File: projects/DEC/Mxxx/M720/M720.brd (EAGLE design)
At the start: 125.7 x 62.2 mm, 38 parts, among them Q1 2N3009, Q2 2N3009, Q3 2N3009, Q4 2N3009, Q5 2N3009, Q6 2N3009

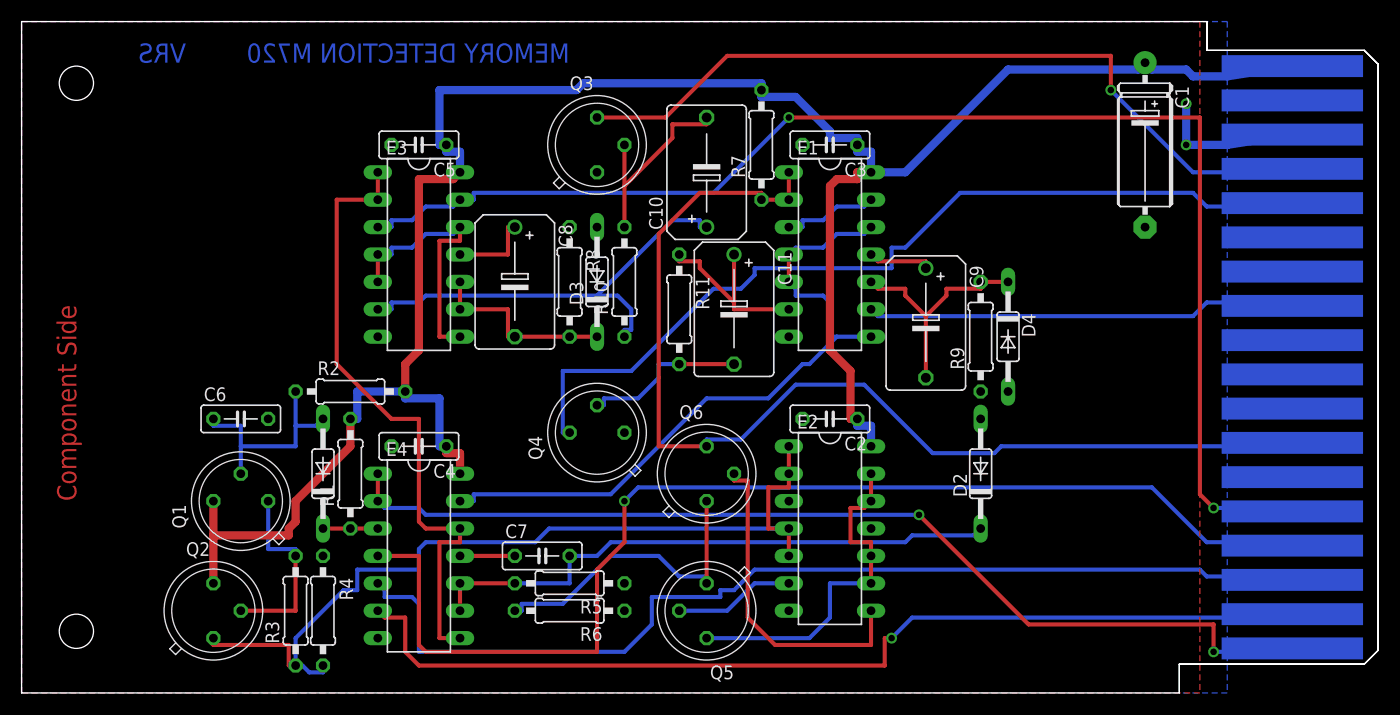
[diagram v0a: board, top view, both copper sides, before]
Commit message: Walk the project tree, making things pass current design rules.
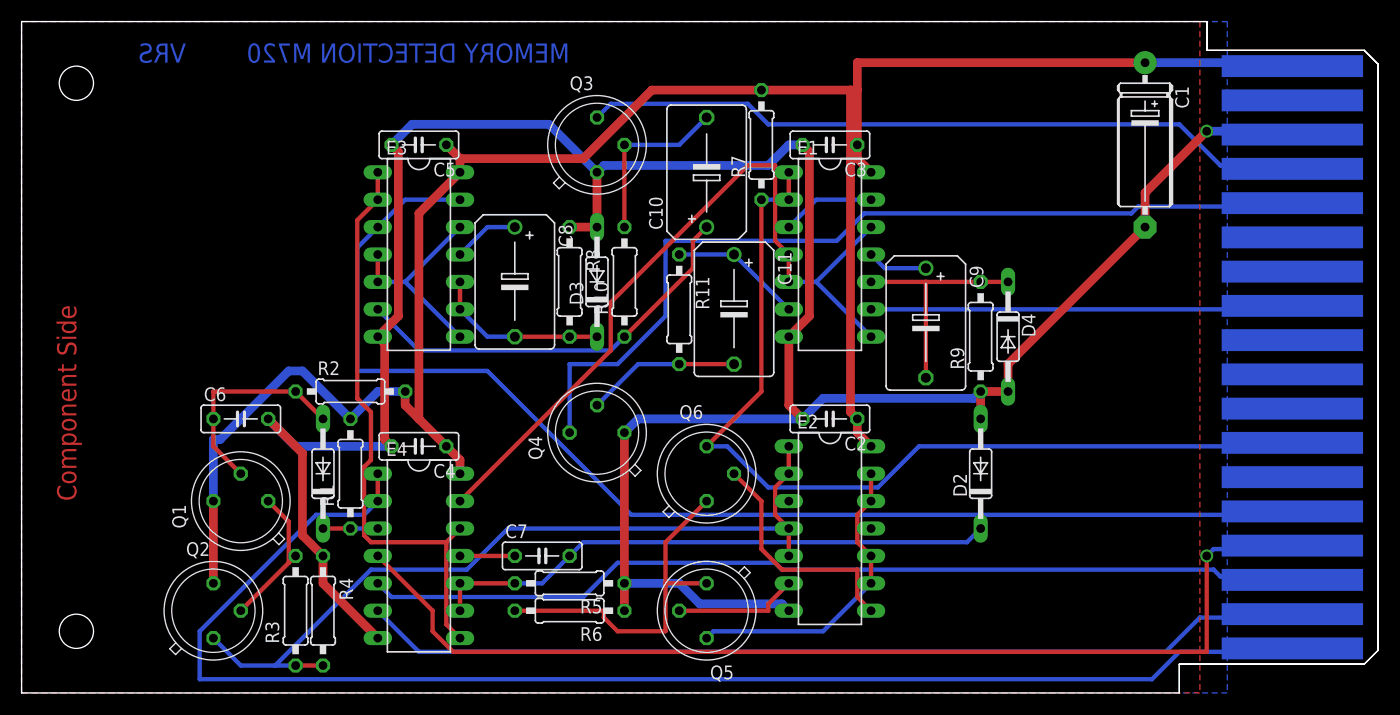
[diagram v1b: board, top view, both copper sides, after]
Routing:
- net GND: track 19.9 -> 255.2 mm, vias 2 -> 1
- net MEM_START: track 94.6 -> 131.0 mm, vias 2 -> 0
- net N$8: track 100.9 -> 87.6 mm
- net N$18: track 125.2 -> 115.1 mm, vias 2 -> 0
- net N$5: track 108.4 -> 98.9 mm
- net N$6: track 95.7 -> 87.3 mm
- net N$20: track 30.3 -> 22.1 mm
- net N$10: track 64.8 -> 72.9 mm
- net N$1: track 82.3 -> 75.3 mm
- net N$19: track 25.6 -> 19.4 mm
- net MEM_DONE: track 73.2 -> 67.5 mm, vias 1 -> 0
- net VCC: track 204.0 -> 198.3 mm
- net N$14: track 17.8 -> 12.3 mm
- net N$16: track 58.9 -> 54.3 mm
- net N$7: track 92.1 -> 87.8 mm, vias 1 -> 0
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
